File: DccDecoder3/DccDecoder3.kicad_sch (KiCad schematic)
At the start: 33 parts, among them J1 PAD, J14 +V, J15 M_OUT_B, J16 M_OUT_A, J17 GND, J2 PAD, J3 0, J4 1, J5 2, J6 3, Q1 DMG2305UX-7, Q2 2N7002K, Q3 2N7002K, Q4 2N7002K, Q5 2N7002K, Q6 2N7002K, SW1 SW_Push, U1 AP7384-33Y, U2 BDR6133, U2 Pico

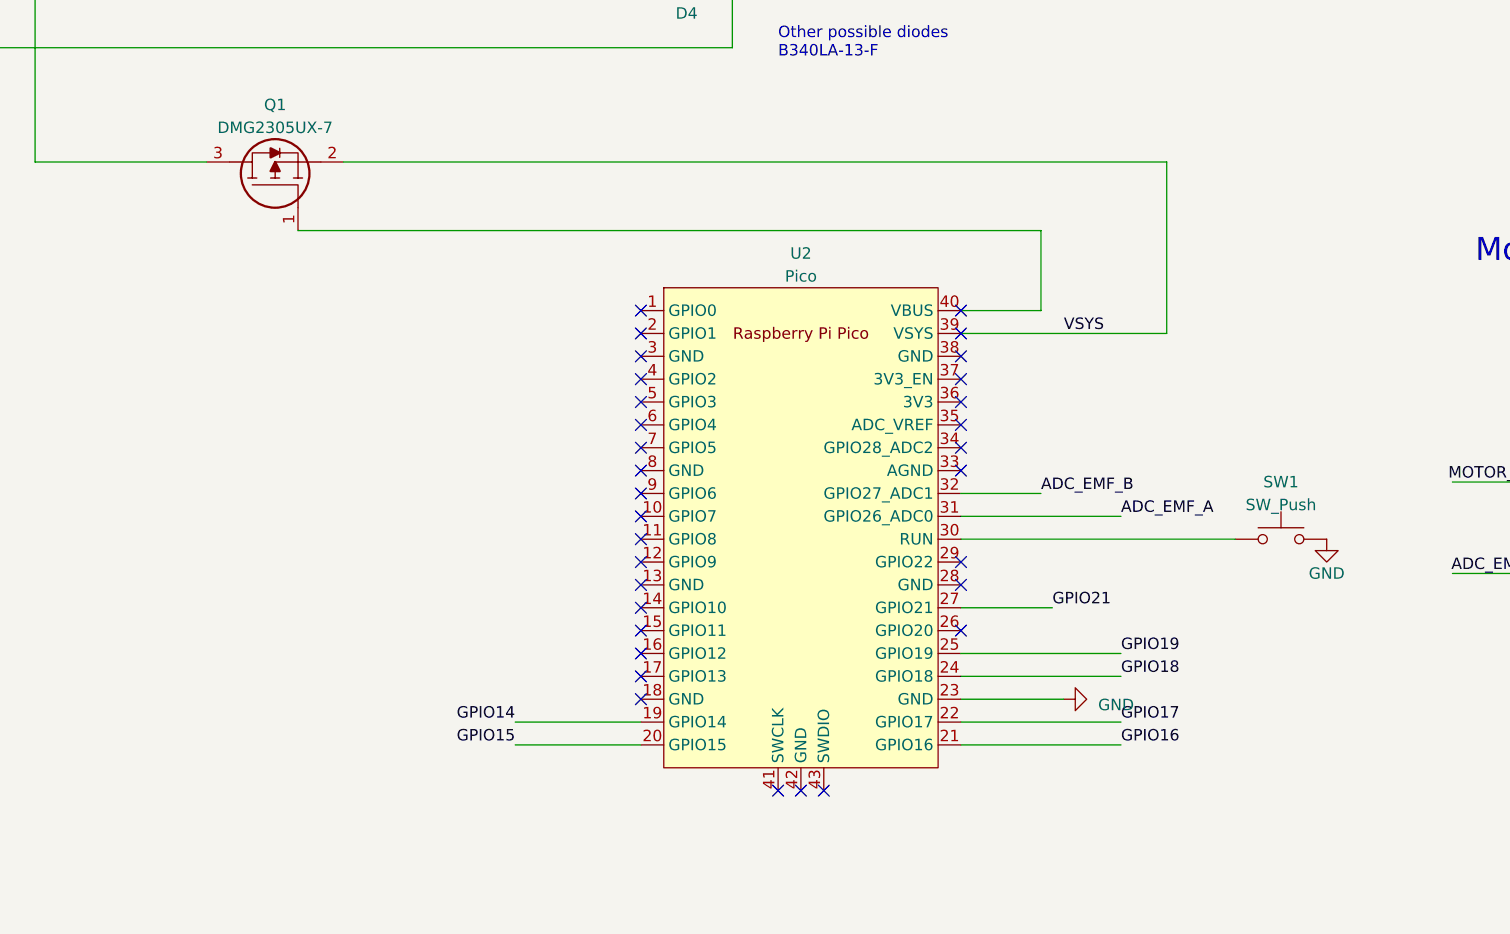
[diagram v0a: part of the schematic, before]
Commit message: 20/01/25 13:46 Titan.local
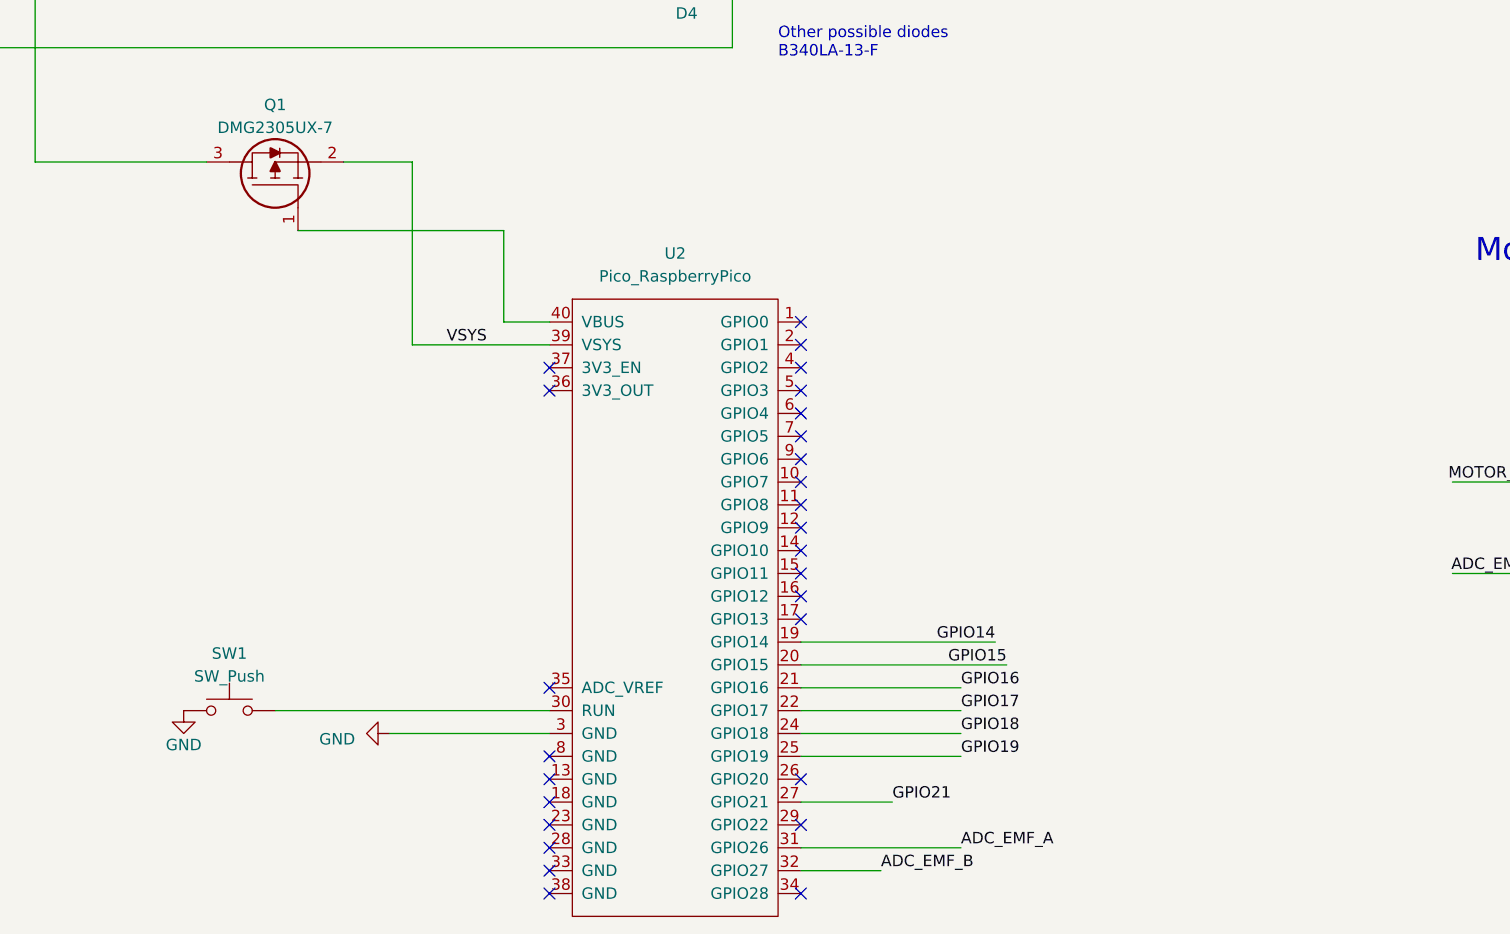
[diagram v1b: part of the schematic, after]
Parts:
- removed U2: Pico, MCU_RaspberryPi_and_Boards:RP2040Pico, symbol MCU_RaspberryPi_and_Boards:Pico
- added U2: Pico_RaspberryPico, PicoNoSwd:RaspberryPico_TH_NoSWD, symbol PicoNoSwd:RaspberryPico-Pico
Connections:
- net ADC_EMF_A: now also U2.31 (GPIO26)
- net ADC_EMF_B: now also U2.32 (GPIO27)
- net GND: now also U2.3 (GND)
- net GPIO14: now also U2.19 (GPIO14)
- net GPIO15: now also U2.20 (GPIO15)
- net GPIO16: now also U2.21 (GPIO16)
- net GPIO17: now also U2.22 (GPIO17)
- net GPIO18: now also U2.24 (GPIO18)
- net GPIO19: now also U2.25 (GPIO19)
- net GPIO21: now also U2.27 (GPIO21)
- net VSYS: now also U2.39 (VSYS)
- net at SW1.1: now also U2.30 (RUN)
- net at Q1.1: now also U2.40 (VBUS)
- no-connect marks 32 -> 27
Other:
- moved on the sheet: SW1
